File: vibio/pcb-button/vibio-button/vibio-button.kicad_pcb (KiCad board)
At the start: 2 copper layers, 114.8 x 41.1 mm, 21 parts, among them J1 Conn_01x03_Female, J2 Conn_01x03_Female, J3 Conn_02x20_Odd_Even, SW1 SW_Push, SW2 SW_Push, SW3 SW_Push, SW4 SW_Push

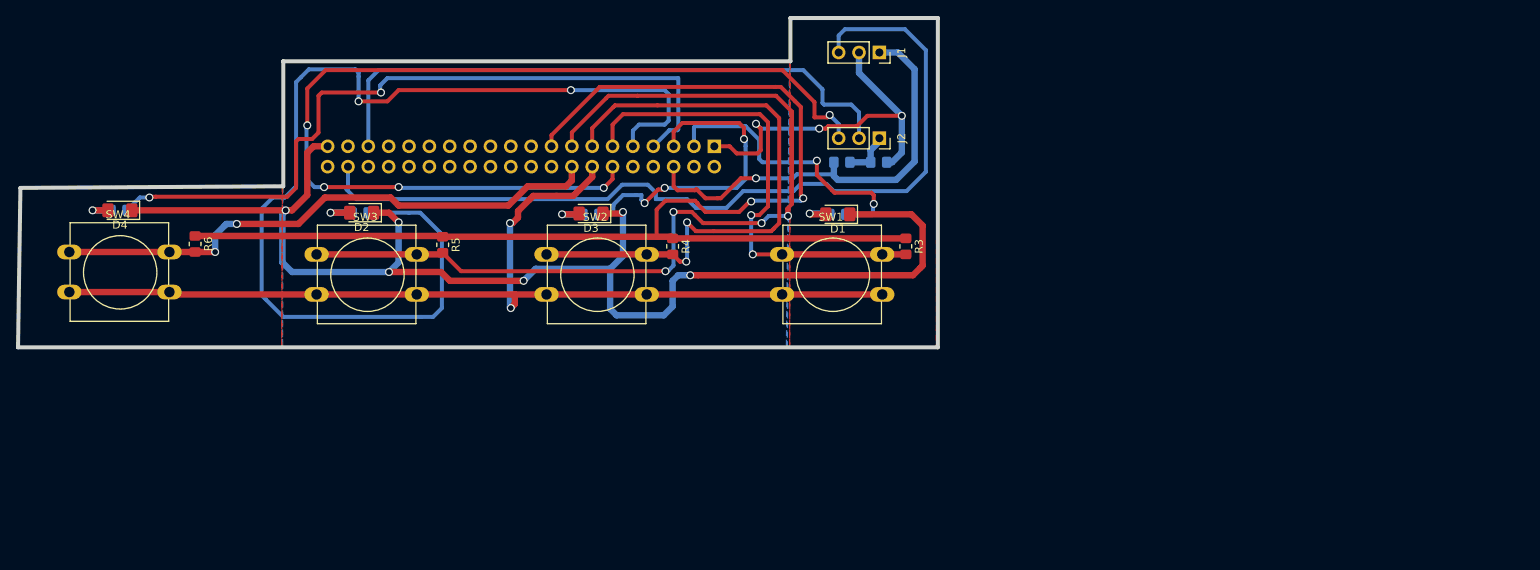
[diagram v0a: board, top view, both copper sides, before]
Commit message: redesign PCB
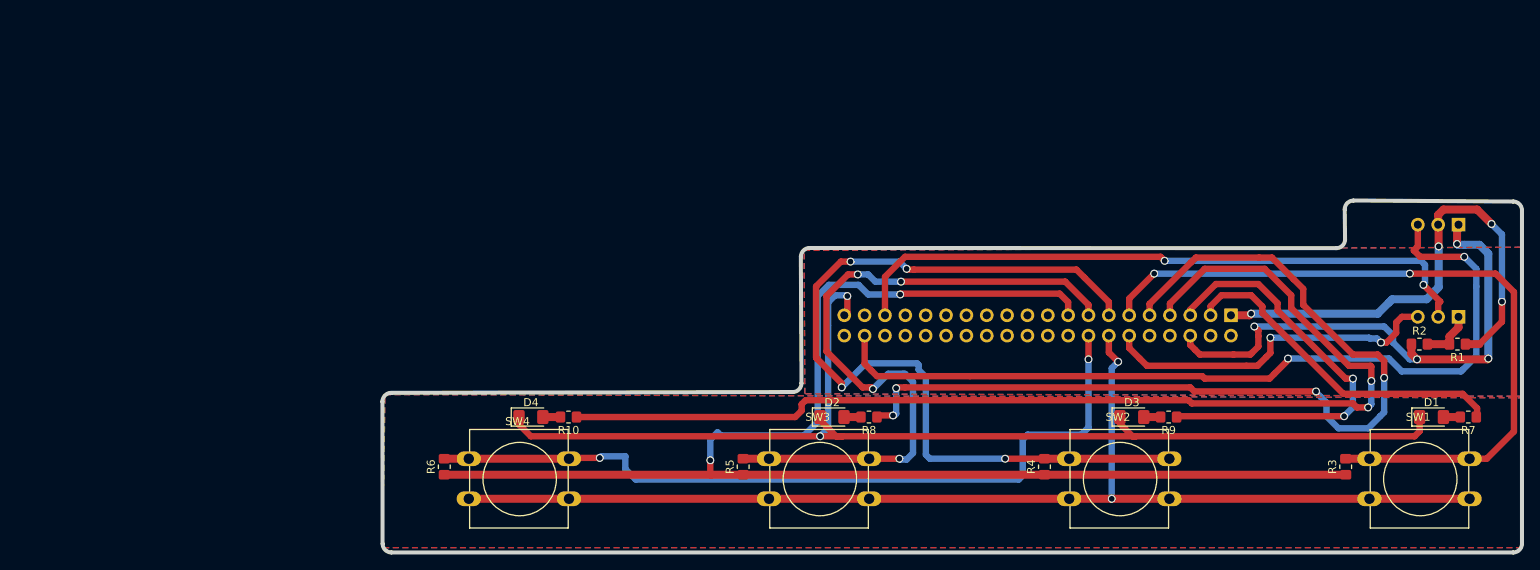
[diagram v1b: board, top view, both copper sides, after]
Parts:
- J1, J2: moved to B.Cu
- R1, R10, R2, R7, R8, R9: moved to F.Cu
- moved R7 82.7 mm to (215.9, 95.6)
- moved D1 78.3 mm to (211.3, 95.6), turned to 0 degrees
- moved SW1 77.6 mm to (203.6, 100.8)
- moved R9 76.4 mm to (178.5, 95.6)
- moved R1 75.7 mm to (214.6, 86.5)
- moved J2 75.6 mm to (214.7, 83.1), turned to 90 degrees
- moved R2 75.6 mm to (209.8, 86.5)
- moved J1 75.4 mm to (214.7, 71.6), turned to 90 degrees
- moved D3 72.1 mm to (173.9, 95.6), turned to 0 degrees
- moved SW2 70.0 mm to (166.1, 100.8)
- moved R8 68.4 mm to (141.1, 95.6)
- moved J3 67.8 mm to (186.3, 82.9)
- moved D2 64.0 mm to (136.5, 95.6), turned to 0 degrees
- moved SW3 62.0 mm to (128.6, 100.8)
- moved R10 61.7 mm to (103.6, 95.6)
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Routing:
- net I2S_SCK: track 125.2 -> 43.4 mm, vias 5 -> 2
- net LED_2: track 92.8 -> 140.2 mm
- net BTN_1: track 75.7 -> 108.6 mm, vias 2 -> 4
- net BTN_0: track 60.2 -> 92.2 mm
- net BTN_3: track 70.2 -> 99.5 mm
- net BTN_2: track 113.0 -> 88.0 mm
- net BTN_VDD: track 159.9 -> 181.7 mm
- net LED_GND: track 164.1 -> 145.9 mm, vias 6 -> 2
- net LED_3: track 134.8 -> 116.7 mm, vias 2 -> 4
- net BTN_GND: track 128.5 -> 146.1 mm
- net I2S_VDD: track 46.1 -> 62.6 mm, vias 3 -> 4
- net LED_1: track 39.6 -> 53.8 mm, vias 3 -> 2
- net I2S_GND: track 54.1 -> 66.9 mm, vias 1 -> 4
- net LED_0: track 37.0 -> 42.4 mm, vias 2 -> 0
- net I2S_WS: track 76.4 -> 81.2 mm, vias 0 -> 2
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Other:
- board size 114.8 x 41.1 mm -> 142.2 x 43.9 mm

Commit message: Ready to Order
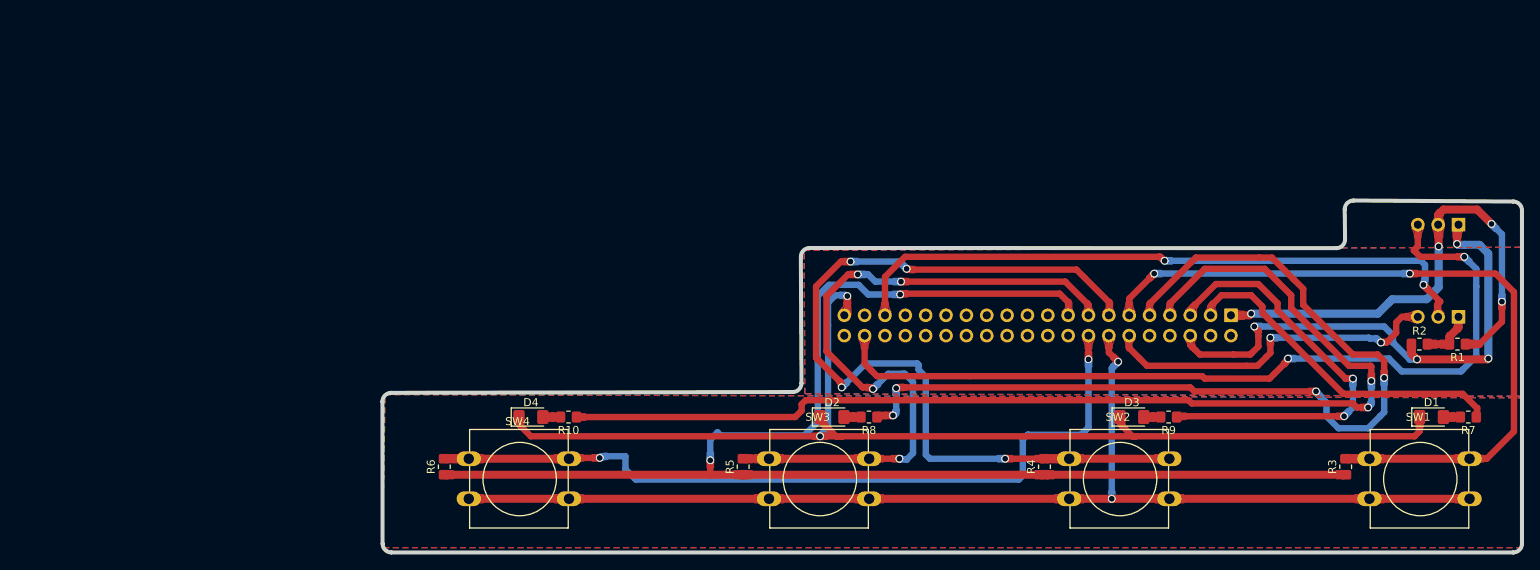
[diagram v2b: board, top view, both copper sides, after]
